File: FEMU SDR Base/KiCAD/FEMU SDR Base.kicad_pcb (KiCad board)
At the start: 4 copper layers, 164.8 x 164.8 mm, 33 parts, among them P2 SDR_Shield_1, P3 SDR_Shield_2, P8 Raspi_Power_Shield, U1 TPS562209, U2 SDR_1_LDO_1_2V, U3 SDR_2_LDO_1_2V, U4 SDR_1_LDO_3_3V, U5 SDR_2_LDO_3_3V

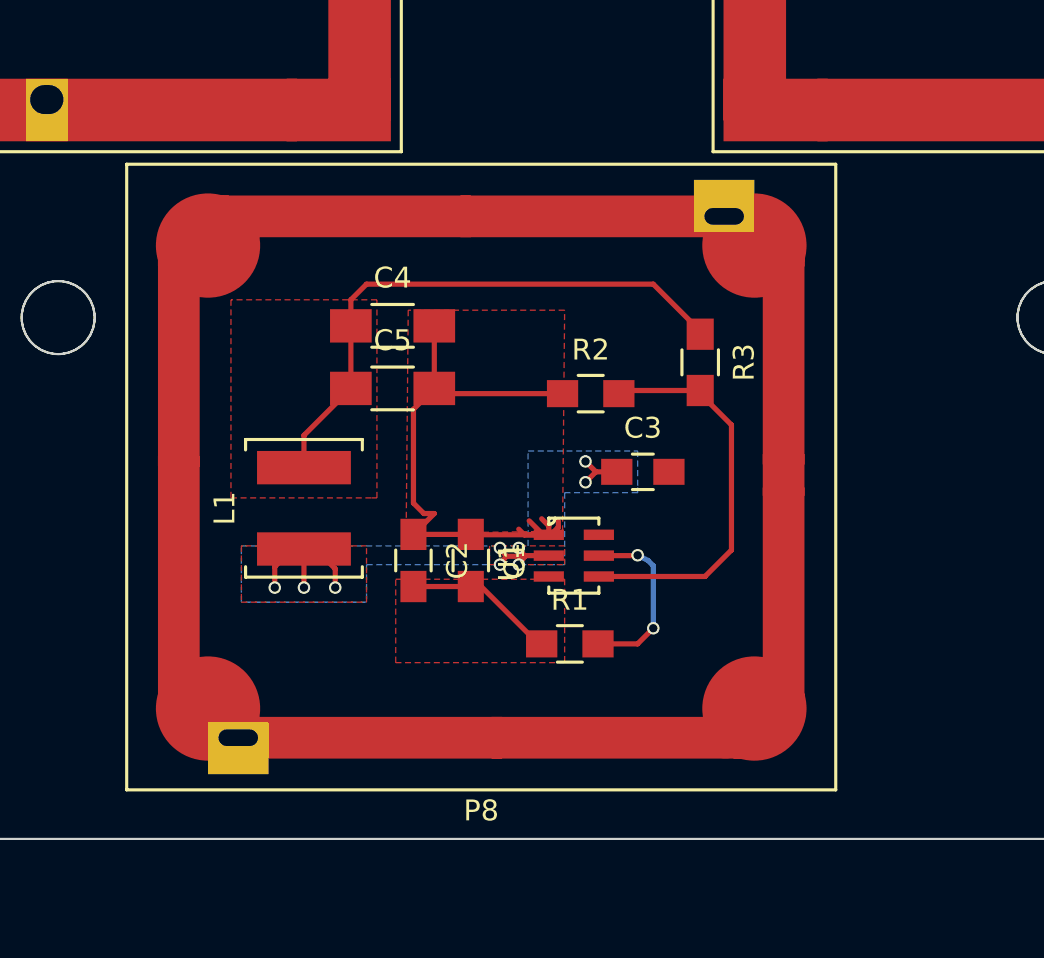
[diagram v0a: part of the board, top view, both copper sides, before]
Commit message: Planning and review
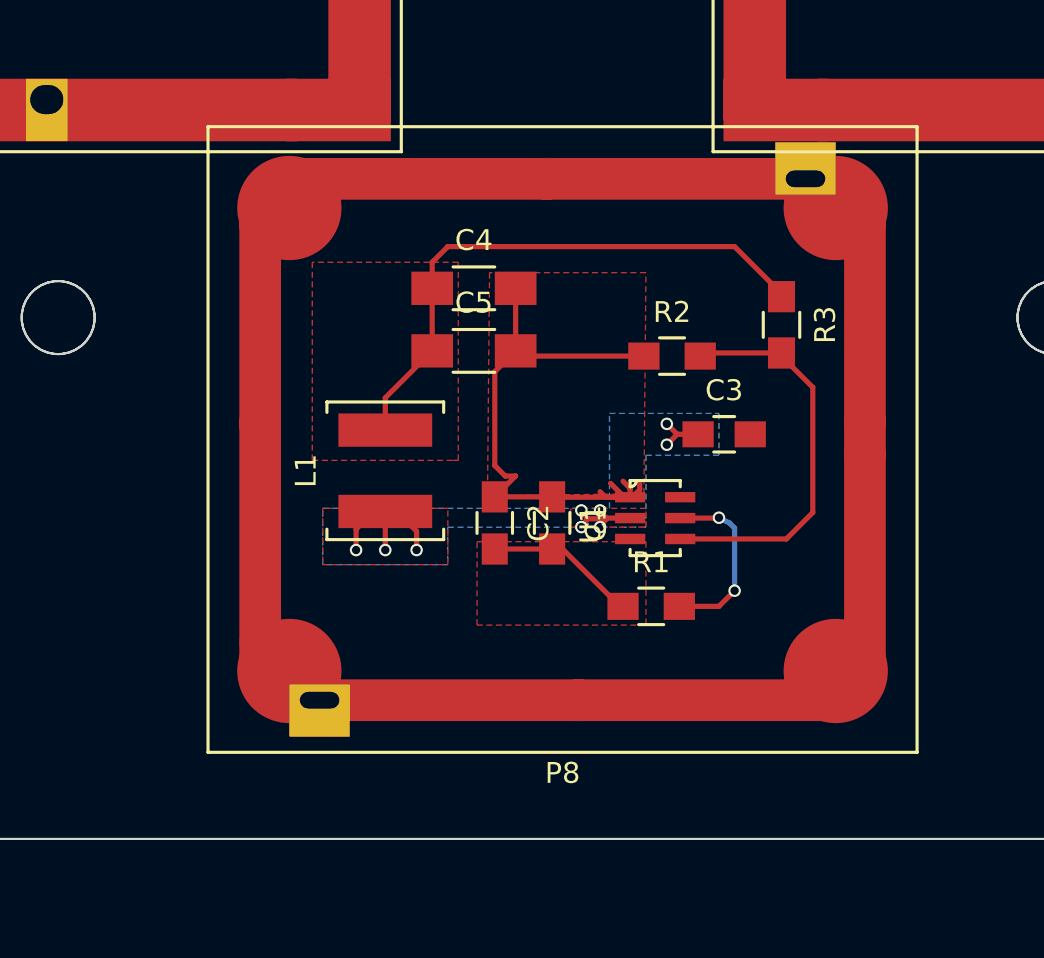
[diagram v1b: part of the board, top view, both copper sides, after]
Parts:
- moved C1 4.30 mm to (84.3, 141.9)
- moved C2 4.30 mm to (81.6, 141.9)
- moved C3 4.30 mm to (92.6, 137.7)
- moved C4 4.30 mm to (80.6, 130.7)
- moved C5 4.30 mm to (80.6, 133.7)
- moved L1 4.30 mm to (76.3, 139.4)
- moved P8 4.30 mm to (84.8, 137.9)
- moved R1 4.30 mm to (89.1, 145.9)
- moved R2 4.30 mm to (90.1, 133.9)
- moved R3 4.30 mm to (95.3, 132.4)
- moved U1 4.30 mm to (89.3, 141.7)
